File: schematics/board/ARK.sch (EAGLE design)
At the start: 208 parts, among them IC2 STM32F103C8T, Q5 8MHz

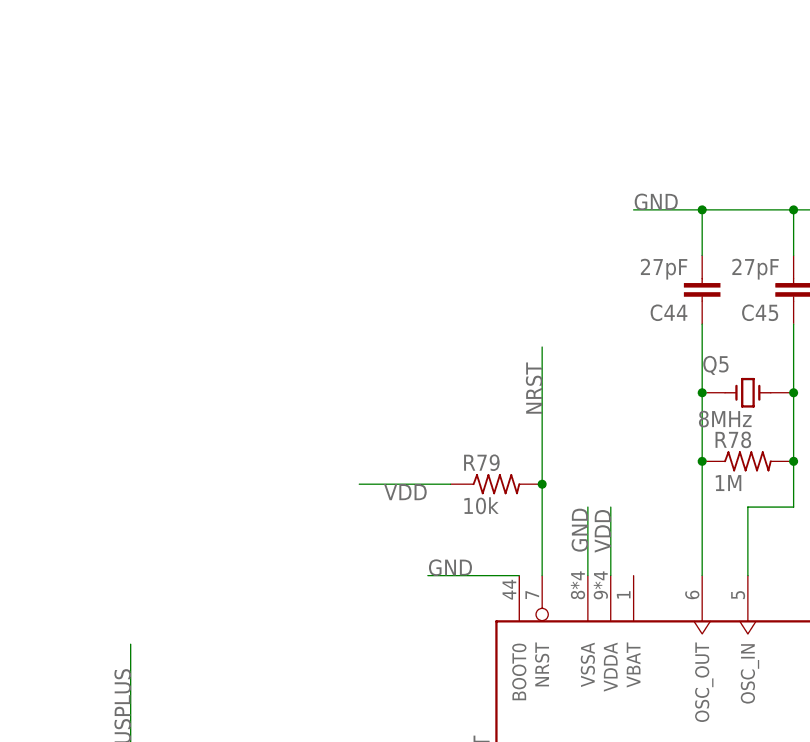
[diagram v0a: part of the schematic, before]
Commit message: Изменения в подключении мк
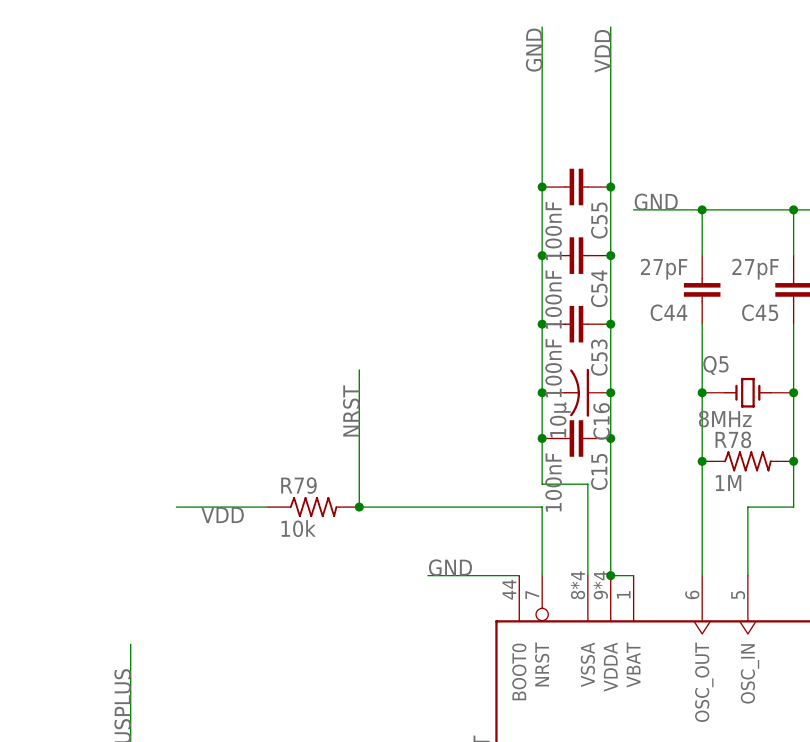
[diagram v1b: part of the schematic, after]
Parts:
- added C15, C53, C54, C55: 100nF, rcl:C-EUC0603
- added C16: 10µ, rcl:C-USC1206
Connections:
- net GND: now also C15.2, C16.2, C53.2, C54.2, C55.2
- net VDD: now also C15.1, C16.1, C53.1, C54.1, C55.1, IC2.VBAT
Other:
- moved on the sheet: R79
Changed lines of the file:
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@@
 <part name="R26" library="resistor" library_urn="urn:adsk.eagle:library:348" deviceset="R-US_" device="R0603" package3d_urn="urn:adsk.eagle:package:23555/3" value="5k1"/>
 <part name="MICRO" library="MicroUSB" deviceset="629105136821" device=""/>
+<part name="C15" library="rcl" library_urn="urn:adsk.eagle:library:334" deviceset="C-EU" device="C0603" package3d_urn="urn:adsk.eagle:package:23616/2" value="100nF"/>
+<part name="C16" library="rcl" library_urn="urn:adsk.eagle:library:334" deviceset="C-US" device="C1206" package3d_urn="urn:adsk.eagle:package:23618/2" value="10µ"/>
+<part name="C53" library="rcl" library_urn="urn:adsk.eagle:library:334" deviceset="C-EU" device="C0603" package3d_urn="urn:adsk.eagle:package:23616/2" value="100nF"/>
+<part name="C54" library="rcl" library_urn="urn:adsk.eagle:library:334" deviceset="C-EU" device="C0603" package3d_urn="urn:adsk.eagle:package:23616/2" value="100nF"/>
+<part name="C55" library="rcl" library_urn="urn:adsk.eagle:library:334" deviceset="C-EU" device="C0603" package3d_urn="urn:adsk.eagle:package:23616/2" value="100nF"/>
 </parts>
 <sheets>
@@
 <instance part="U$26" gate="G$1" x="58.42" y="43.18" smashed="yes"/>
 <instance part="U$1" gate="G$1" x="241.3" y="50.8" smashed="yes"/>
-<instance part="R79" gate="G$1" x="462.28" y="378.46" smashed="yes">
-<attribute name="NAME" x="458.47" y="379.9586" size="1.778" layer="95"/>
-<attribute name="VALUE" x="458.47" y="375.158" size="1.778" layer="96"/>
+<instance part="R79" gate="G$1" x="441.96" y="375.92" smashed="yes">
+<attribute name="NAME" x="438.15" y="377.4186" size="1.778" layer="95"/>
+<attribute name="VALUE" x="438.15" y="372.618" size="1.778" layer="96"/>
 </instance>
 <instance part="LED3" gate="G$1" x="297.18" y="292.1" smashed="yes" rot="R270">
@@
 <attribute name="VALUE" x="508" y="226.06" size="1.778" layer="96"/>
 </instance>
+<instance part="C15" gate="G$1" x="472.44" y="383.54" smashed="yes" rot="R270">
+<attribute name="NAME" x="472.821" y="382.016" size="1.778" layer="95" rot="R270"/>
+<attribute name="VALUE" x="467.741" y="382.016" size="1.778" layer="96" rot="R270"/>
+</instance>
+<instance part="C16" gate="G$1" x="472.44" y="388.62" smashed="yes" rot="R270">
+<attribute name="NAME" x="473.075" y="387.604" size="1.778" layer="95" rot="R270"/>
+<attribute name="VALUE" x="468.249" y="387.604" size="1.778" layer="96" rot="R270"/>
+</instance>
+<instance part="C53" gate="G$1" x="472.44" y="396.24" smashed="yes" rot="R270">
+<attribute name="NAME" x="472.821" y="394.716" size="1.778" layer="95" rot="R270"/>
+<attribute name="VALUE" x="467.741" y="394.716" size="1.778" layer="96" rot="R270"/>
+</instance>
+<instance part="C54" gate="G$1" x="472.44" y="403.86" smashed="yes" rot="R270">
+<attribute name="NAME" x="472.821" y="402.336" size="1.778" layer="95" rot="R270"/>
+<attribute name="VALUE" x="467.741" y="402.336" size="1.778" layer="96" rot="R270"/>
+</instance>
+<instance part="C55" gate="G$1" x="472.44" y="411.48" smashed="yes" rot="R270">
+<attribute name="NAME" x="472.821" y="409.956" size="1.778" layer="95" rot="R270"/>
+<attribute name="VALUE" x="467.741" y="409.956" size="1.778" layer="96" rot="R270"/>
+</instance>
 </instances>
 <busses>
@@
 </segment>
 <segment>
-<wire x1="472.44" y1="368.3" x2="472.44" y2="375.92" width="0.1524" layer="91"/>
-<label x="472.44" y="370.84" size="1.778" layer="95" rot="R90"/>
+<wire x1="472.44" y1="368.3" x2="472.44" y2="378.46" width="0.1524" layer="91"/>
+<label x="467.36" y="424.18" size="1.778" layer="95" rot="R90"/>
 <pinref part="IC2" gate="MCU" pin="VSSA"/>
+<wire x1="472.44" y1="378.46" x2="467.36" y2="378.46" width="0.1524" layer="91"/>
+<wire x1="467.36" y1="378.46" x2="467.36" y2="383.54" width="0.1524" layer="91"/>
+<pinref part="C15" gate="G$1" pin="2"/>
+<wire x1="467.36" y1="383.54" x2="467.36" y2="388.62" width="0.1524" layer="91"/>
+<junction x="467.36" y="383.54"/>
+<pinref part="C16" gate="G$1" pin="2"/>
+<wire x1="467.36" y1="388.62" x2="467.36" y2="396.24" width="0.1524" layer="91"/>
+<junction x="467.36" y="388.62"/>
+<pinref part="C53" gate="G$1" pin="2"/>
+<wire x1="467.36" y1="396.24" x2="467.36" y2="403.86" width="0.1524" layer="91"/>
+<junction x="467.36" y="396.24"/>
+<pinref part="C54" gate="G$1" pin="2"/>
+<wire x1="467.36" y1="403.86" x2="467.36" y2="411.48" width="0.1524" layer="91"/>
+<junction x="467.36" y="403.86"/>
+<pinref part="C55" gate="G$1" pin="2"/>
+<wire x1="467.36" y1="411.48" x2="467.36" y2="429.26" width="0.1524" layer="91"/>
+<junction x="467.36" y="411.48"/>
 </segment>
 <segment>
@@
 </segment>
 <segment>
-<wire x1="474.98" y1="368.3" x2="474.98" y2="375.92" width="0.1524" layer="91"/>
-<label x="474.98" y="370.84" size="1.778" layer="95" rot="R90"/>
+<wire x1="474.98" y1="368.3" x2="474.98" y2="383.54" width="0.1524" layer="91"/>
+<label x="474.98" y="424.18" size="1.778" layer="95" rot="R90"/>
 <pinref part="IC2" gate="MCU" pin="VDDA"/>
+<pinref part="C15" gate="G$1" pin="1"/>
+<wire x1="474.98" y1="383.54" x2="474.98" y2="388.62" width="0.1524" layer="91"/>
+<junction x="474.98" y="383.54"/>
+<pinref part="C16" gate="G$1" pin="1"/>
+<wire x1="474.98" y1="388.62" x2="474.98" y2="396.24" width="0.1524" layer="91"/>
+<junction x="474.98" y="388.62"/>
+<pinref part="C53" gate="G$1" pin="1"/>
+<wire x1="474.98" y1="396.24" x2="474.98" y2="403.86" width="0.1524" layer="91"/>
+<junction x="474.98" y="396.24"/>
+<pinref part="C54" gate="G$1" pin="1"/>
+<wire x1="474.98" y1="403.86" x2="474.98" y2="411.48" width="0.1524" layer="91"/>
+<junction x="474.98" y="403.86"/>
+<pinref part="C55" gate="G$1" pin="1"/>
+<wire x1="474.98" y1="411.48" x2="474.98" y2="429.26" width="0.1524" layer="91"/>
+<junction x="474.98" y="411.48"/>
+<pinref part="IC2" gate="MCU" pin="VBAT"/>
+<wire x1="477.52" y1="368.3" x2="474.98" y2="368.3" width="0.1524" layer="91"/>
+<junction x="474.98" y="368.3"/>
 </segment>
 <segment>
@@
 </segment>
 <segment>
-<wire x1="457.2" y1="378.46" x2="447.04" y2="378.46" width="0.1524" layer="91"/>
-<label x="454.66" y="378.46" size="1.778" layer="95" rot="R180"/>
+<wire x1="436.88" y1="375.92" x2="426.72" y2="375.92" width="0.1524" layer="91"/>
+<label x="434.34" y="375.92" size="1.778" layer="95" rot="R180"/>
 <pinref part="R79" gate="G$1" pin="1"/>
 </segment>
@@
 <net name="NRST" class="0">
 <segment>
-<wire x1="467.36" y1="368.3" x2="467.36" y2="378.46" width="0.1524" layer="91"/>
 <pinref part="R79" gate="G$1" pin="2"/>
-<wire x1="467.36" y1="378.46" x2="467.36" y2="393.7" width="0.1524" layer="91"/>
-<junction x="467.36" y="378.46"/>
-<label x="467.36" y="386.08" size="1.778" layer="95" rot="R90"/>
+<wire x1="447.04" y1="375.92" x2="447.04" y2="391.16" width="0.1524" layer="91"/>
+<label x="447.04" y="383.54" size="1.778" layer="95" rot="R90"/>
 <pinref part="IC2" gate="MCU" pin="NRST"/>
+<wire x1="447.04" y1="375.92" x2="467.36" y2="375.92" width="0.1524" layer="91"/>
+<wire x1="467.36" y1="375.92" x2="467.36" y2="368.3" width="0.1524" layer="91"/>
+<junction x="447.04" y="375.92"/>
 </segment>
 <segment>
